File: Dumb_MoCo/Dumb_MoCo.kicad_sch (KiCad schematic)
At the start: 17 parts, among them U1 VNH7070AS

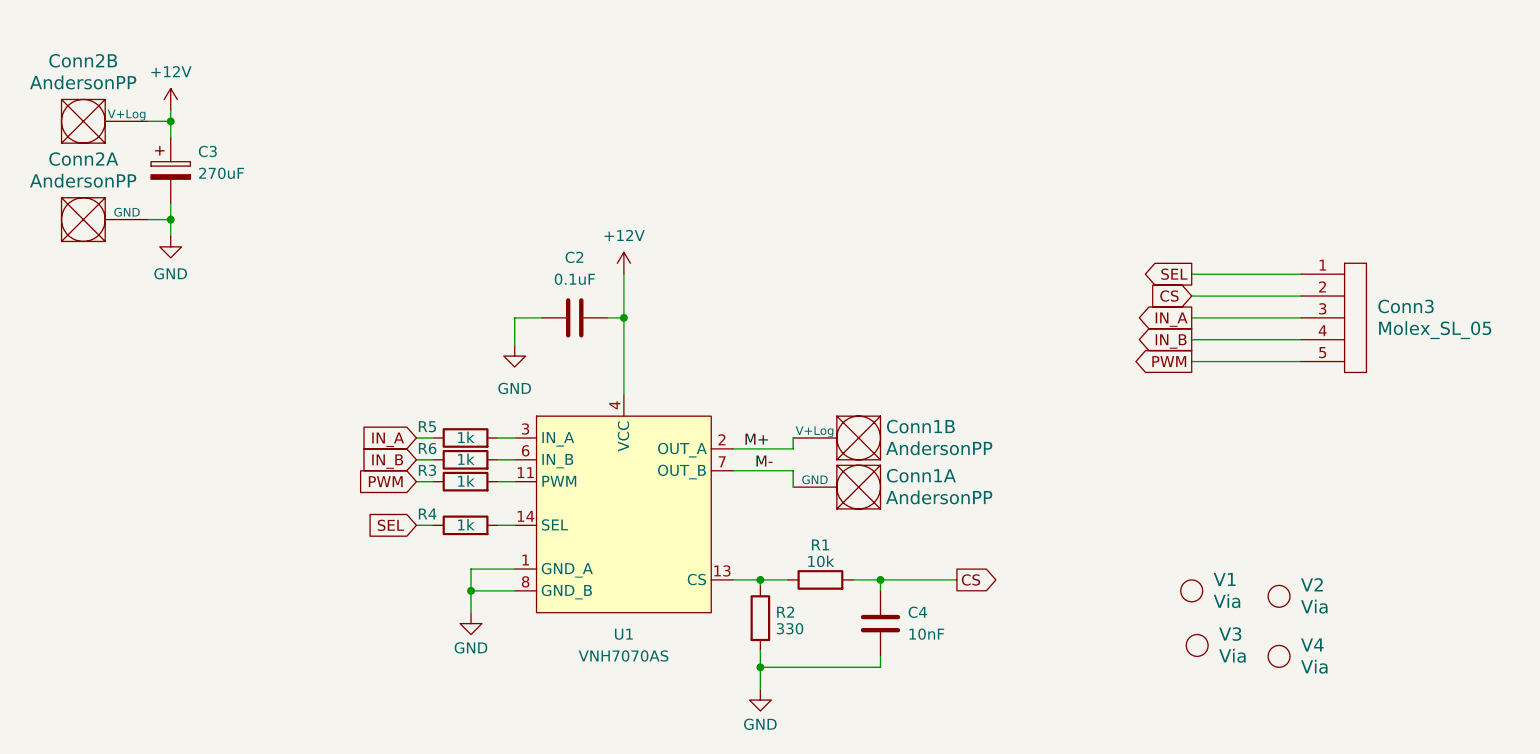
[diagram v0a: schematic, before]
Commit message: Added Chamber Ult Silkscreen
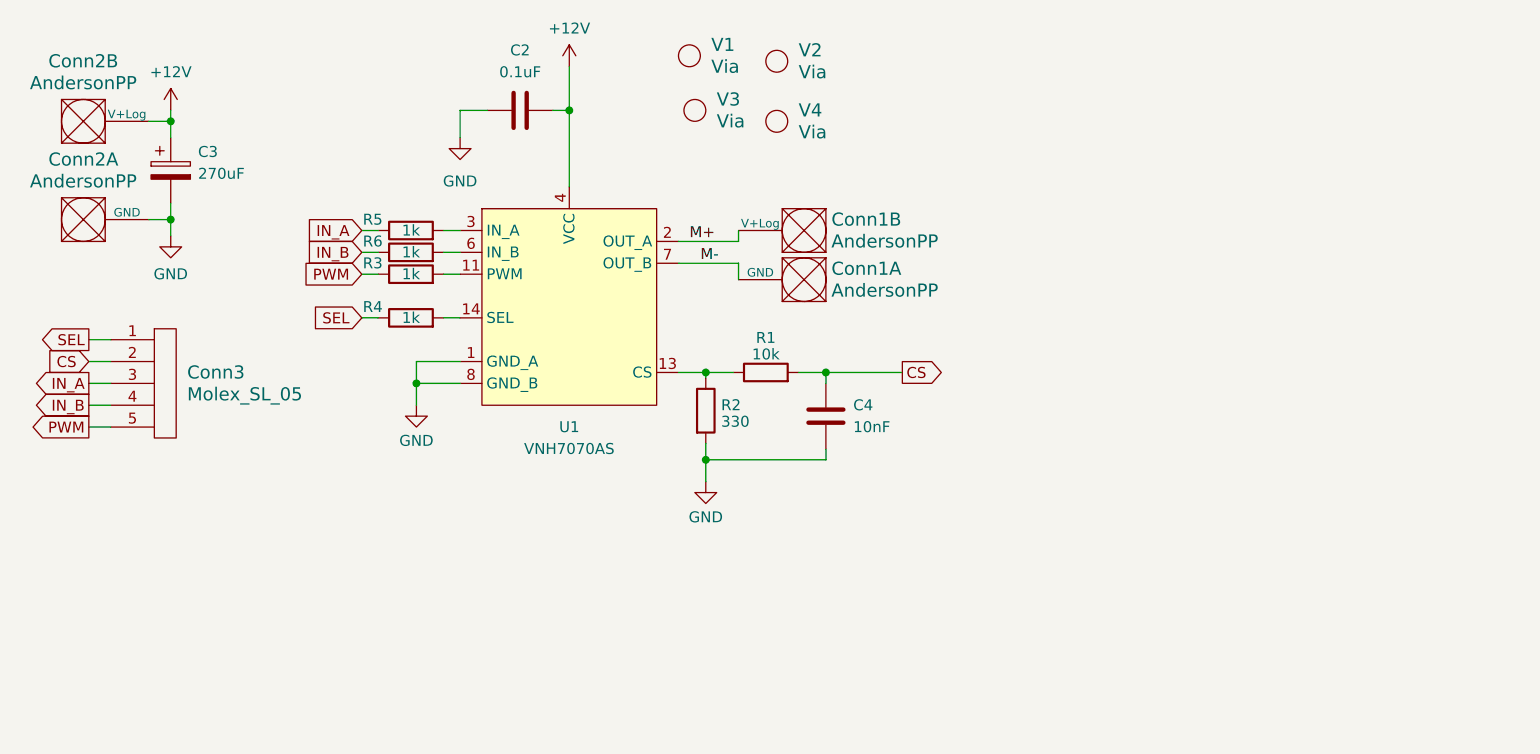
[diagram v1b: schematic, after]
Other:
- moved on the sheet: C2, C4, Conn1A, Conn1B, Conn3, R1, R2, R3, R4, R5, R6, U1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
